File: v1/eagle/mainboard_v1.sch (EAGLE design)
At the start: 8 parts

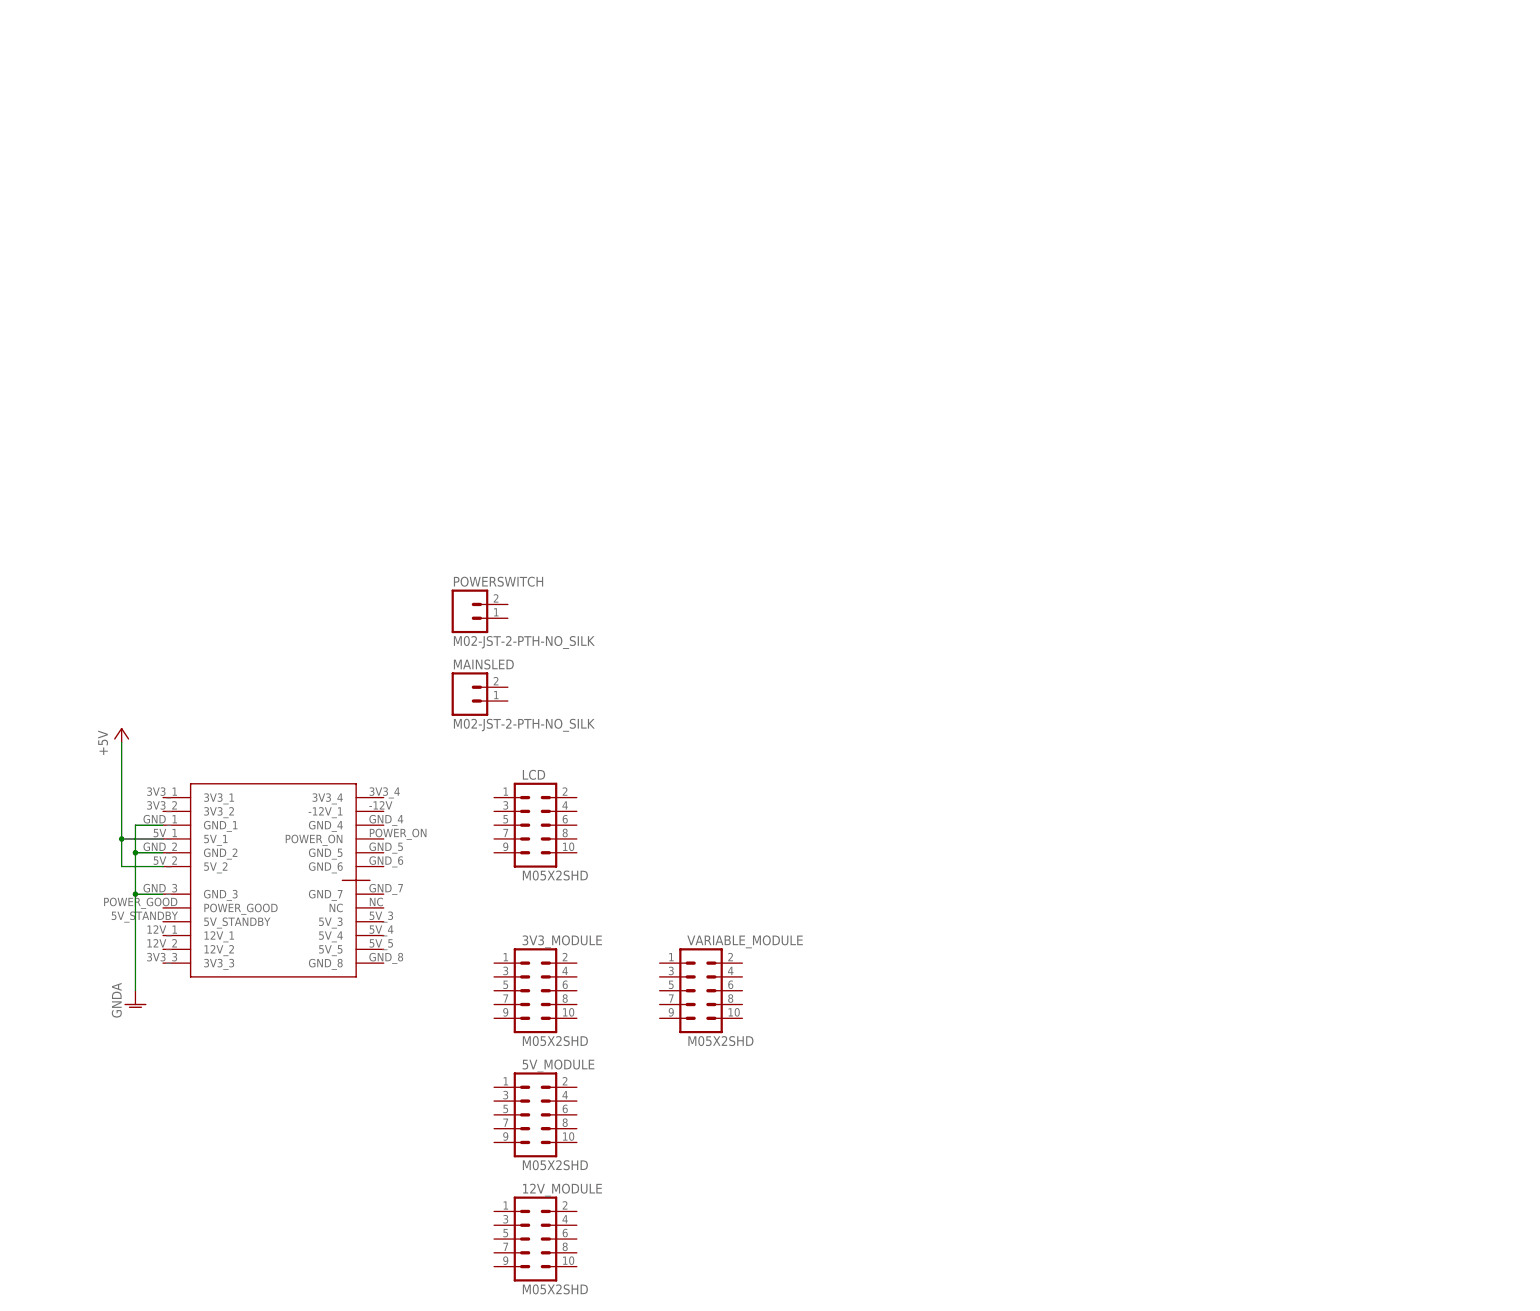
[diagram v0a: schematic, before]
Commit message: mainboard is all laid out
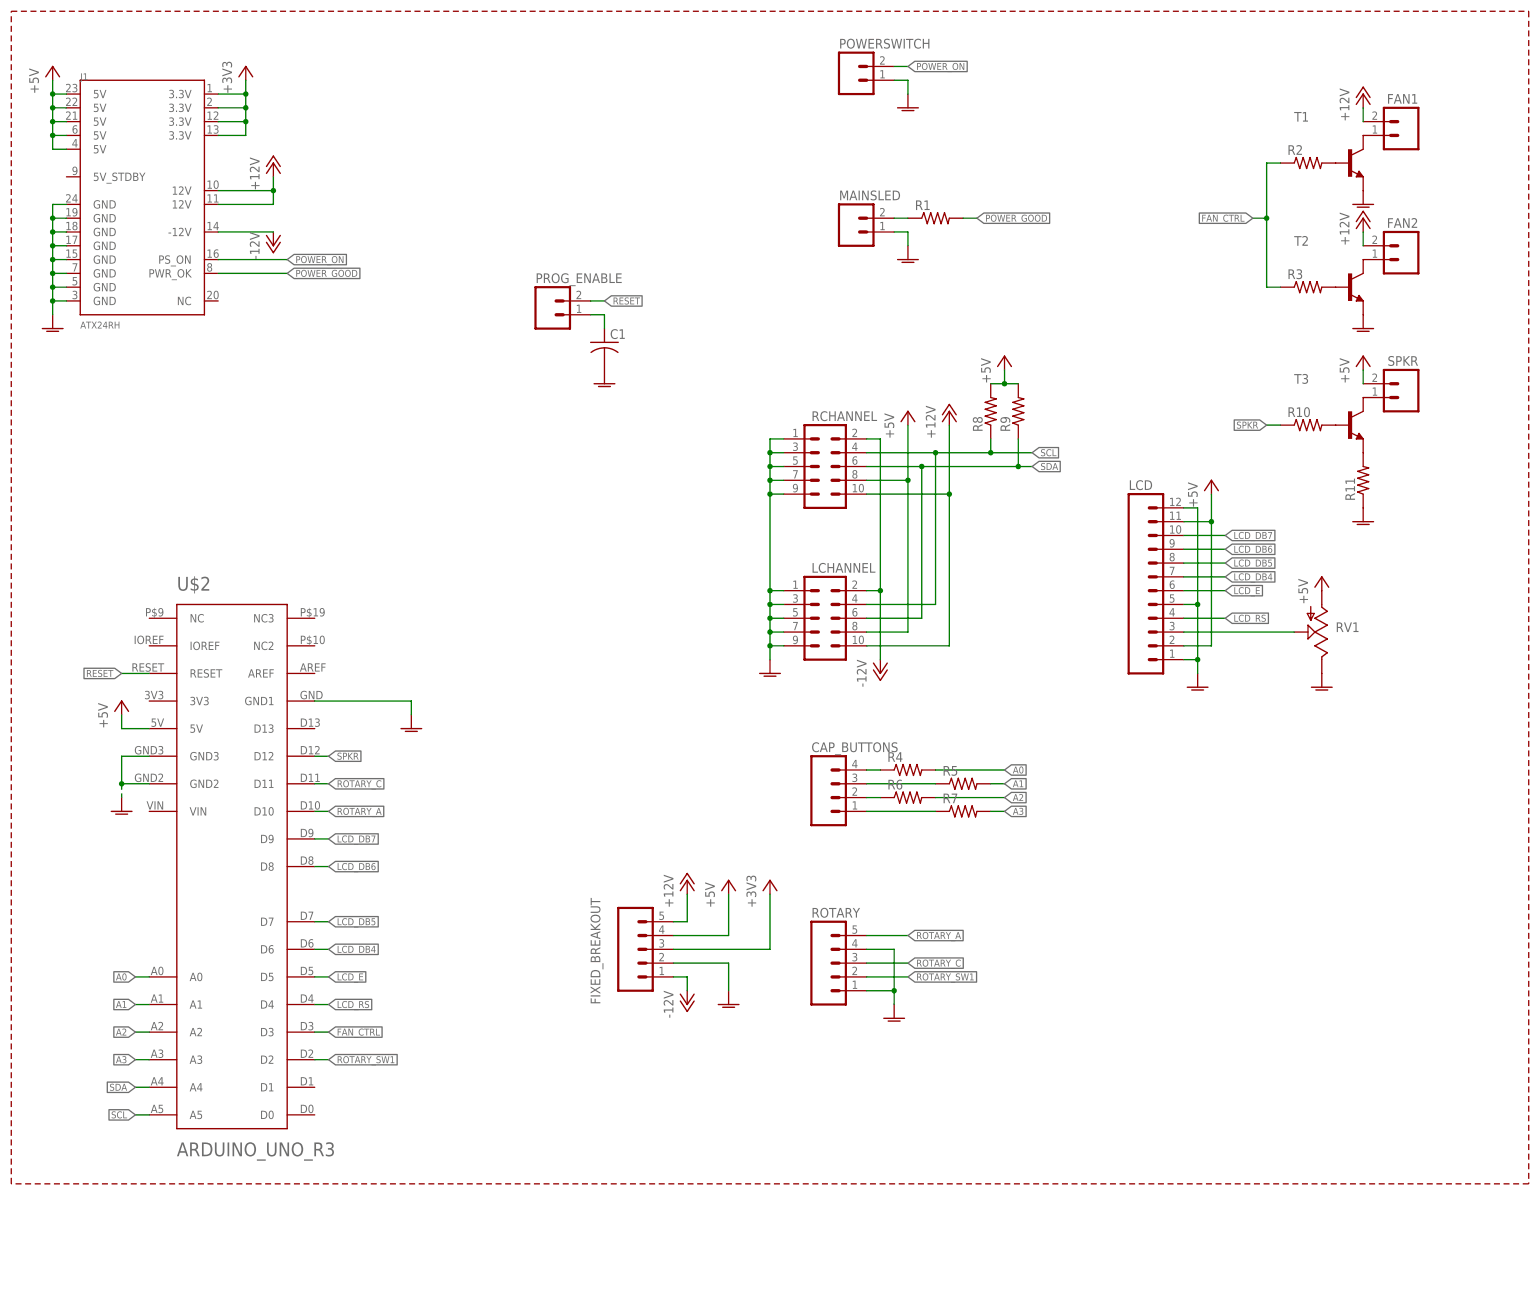
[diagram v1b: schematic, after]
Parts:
- removed 12V_MODULE, 3V3_MODULE, 5V_MODULE, VARIABLE_MODULE: M05X2SHD, SparkFun-Connectors:M05X2SHD
- removed U$1: ATX-PSU-24, parts:ATX-PSU-24
- added C1: (no value), rcl:C-USC0805
- added CAP_BUTTONS: (no value), con-amp-quick:M04
- added FAN1, FAN2, PROG_ENABLE, SPKR: M02PTH, SparkFun-Connectors:M02PTH
- added FIXED_BREAKOUT, ROTARY: (no value), con-amp-quick:M05
- added J1: ATX24RH, SparkFun-Connectors:ATX24RH
- added LCHANNEL, RCHANNEL: M05X2SHD, SparkFun-Connectors:M05X2SHD
- added R1, R10, R11, R2, R3, R4, R5, R6, R7, R8, R9: (no value), rcl:R-US_R0805
- added RV1: (no value), SparkFun-Electromechanical:POTTRIM
- added T1, T2, T3: (no value), transistor:MMBT2222ALT1-NPN-SOT23-BEC
- added U$2: ARDUINO_UNO_R3, parts:ARDUINO_UNO_R3
- LCD: value M05X2SHD -> (none); device SparkFun-Connectors:M05X2SHD -> con-amp-quick:M12
- MAINSLED, POWERSWITCH: value M02-JST-2-PTH-NO_SILK -> M02PTH; device SparkFun-Connectors:M02-JST-2-PTH-NO_SILK -> SparkFun-Connectors:M02PTH
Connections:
- new net +12V: FAN1.2, FAN2.2, FIXED_BREAKOUT.5, J1.12V@0, J1.12V@1, LCHANNEL.10, RCHANNEL.10
- new net +3V3: FIXED_BREAKOUT.3, J1.3.3V@0, J1.3.3V@1, J1.3.3V@2, J1.3.3V@3
- new net -12V: FIXED_BREAKOUT.1, J1.-12V, LCHANNEL.2, RCHANNEL.2
- new net A0: R4.2, U$2.A0
- new net A1: R5.2, U$2.A1
- new net A2: R6.2, U$2.A2
- new net A3: R7.2, U$2.A3
- new net FAN_CTRL: R2.1, R3.1, U$2.D3
- new net LCD_DB4: LCD.7, U$2.D6
- new net LCD_DB5: LCD.8, U$2.D7
- new net LCD_DB6: LCD.9, U$2.D8
- new net LCD_DB7: LCD.10, U$2.D9
- new net LCD_E: LCD.6, U$2.D5
- new net LCD_RS: LCD.4, U$2.D4
- new net N$1: R2.2, T1.B
- new net N$11: CAP_BUTTONS.4, R4.1
- new net N$12: CAP_BUTTONS.3, R5.1
- new net N$13: CAP_BUTTONS.2, R6.1
- new net N$14: CAP_BUTTONS.1, R7.1
- new net N$15: SPKR.1, T3.C
- new net N$16: R10.2, T3.B
- new net N$17: R11.2, T3.E
- new net N$19: C1.1, PROG_ENABLE.1
- new net N$2: MAINSLED.2, R1.1
- new net N$3: R3.2, T2.B
- new net N$4: FAN1.1, T1.C
- new net N$5: FAN2.1, T2.C
- new net N$6: LCD.3, RV1.S
- new net POWER_GOOD: J1.PWR_OK, R1.2
- new net POWER_ON: J1.PS_ON, POWERSWITCH.2
- new net RESET: PROG_ENABLE.2, U$2.RESET
- new net ROTARY_A: ROTARY.5, U$2.D10
- new net ROTARY_C: ROTARY.3, U$2.D11
- new net ROTARY_SW1: ROTARY.2, U$2.D2
- new net SCL: LCHANNEL.4, R8.1, RCHANNEL.4, U$2.A5
- new net SDA: LCHANNEL.6, R9.1, RCHANNEL.6, U$2.A4
- new net SPKR: R10.1, U$2.D12
- net +5V: now also FIXED_BREAKOUT.4, J1.5V@0, J1.5V@1, J1.5V@2, J1.5V@3, J1.5V@4, LCD.11, LCD.2, LCHANNEL.8, R8.2, R9.2, RCHANNEL.8, RV1.A, SPKR.2, U$2.5V; no longer U$1.5V_1, U$1.5V_2
- net GNDA: now also C1.2, FIXED_BREAKOUT.2, J1.GND@0, J1.GND@1, J1.GND@2, J1.GND@3, J1.GND@4, J1.GND@5, J1.GND@6, J1.GND@7, LCD.1, LCD.12, LCD.5, LCHANNEL.1, LCHANNEL.3, LCHANNEL.5, LCHANNEL.7, LCHANNEL.9, MAINSLED.1, POWERSWITCH.1, R11.1, RCHANNEL.1, RCHANNEL.3, RCHANNEL.5, RCHANNEL.7, RCHANNEL.9, ROTARY.1, ROTARY.4, RV1.E, T1.E, T2.E, U$2.GND1, U$2.GND2, U$2.GND3; no longer U$1.GND_1, U$1.GND_2, U$1.GND_3
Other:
- moved on the sheet: MAINSLED, POWERSWITCH

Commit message: outstanding work
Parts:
- removed CAP_BUTTONS: (no value), con-amp-quick:M04
- removed FIXED_BREAKOUT: (no value), con-amp-quick:M05
- removed MAINSLED, POWERSWITCH: M02PTH, SparkFun-Connectors:M02PTH
- removed R4, R5, R6, R7: (no value), rcl:R-US_R0805
- removed RV1: (no value), SparkFun-Electromechanical:POTTRIM
- removed T1, T2, T3: (no value), transistor:MMBT2222ALT1-NPN-SOT23-BEC
- added -12V_OUT, 12V_OUT, 3V3_OUT, 5V_OUT, GND_FIX: TPPAD1-20, testpad:TPPAD1-20
- added CH1, CH2: (no value), led:LED5MM
- added I2C_EXTRA, JP1: M05X2NO_SILK, SparkFun-Connectors:M05X2NO_SILK
- added LD1, LD2, LD3, LD4: (no value), led:DUOLED-RG-A
- added PWRGOOD, PWRSW, STANDBY: M02PTH, SparkFun-Connectors:M02PTH
- added Q1, Q2, QA1, QA2, QA3, QB1, QB2, QB3, QC1, QC2, QC3, QD1, QD2, QD3: 2N7002L, parts:2N7002L
- added QD4, QD5: BSS84, transistor-small-signal:BSS84
- added R12, RB1, RB2, RB3, RB4, RC1, RC2, RC3, RC4, RD1, RD2, RD3, RD4, RD5: (no value), rcl:R-US_R0805
- added R13: 1R1 10W, resistor-power:RMNS-5
- added RA1: 10k, rcl:R-US_R0805
- added RA2: 470, rcl:R-US_R0805
- added RA3, RA4: 1M, rcl:R-US_R0805
- added U$1, U$3, U$4, U$5: MF-R300, parts:MF-R300
- added U$10, U$6, U$8, U$9: SPST, parts:SPST
- LCD: device con-amp-quick:M12 -> con-amp-quick:M04
- U$2: value ARDUINO_UNO_R3 -> ARDUINO_UNO_R3MINIMUM; device parts:ARDUINO_UNO_R3 -> parts:ARDUINO_UNO_R3MINIMUM
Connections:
- removed net A2: R6.2, U$2.A2
- removed net A3: R7.2, U$2.A3
- removed net N$11: CAP_BUTTONS.4, R4.1
- removed net N$12: CAP_BUTTONS.3, R5.1
- removed net N$6: LCD.3, RV1.S
- new net 5V_OUT: 5V_OUT.TP, QB2.G, QB3.G, RB4.1, U$3.2
- new net 5V_OUT1: 3V3_OUT.TP, QC2.G, QC3.G, RC4.1, U$4.2
- new net 5V_STANDBY: J1.5V_STDBY, R1.2
- new net CH1_SW: CH1.C, U$2.A3
- new net CH2_SW: CH2.C, U$2.A2
- new net D13: JP1.1, U$2.D13
- new net N$18: PWRGOOD.2, R12.1
- new net N$20: RA1.1, U$1.2, U$6.P$2
- new net N$21: LD3.CR, QC1.D
- new net N$22: LD3.A, RC2.1
- new net N$23: LD3.CG, QC2.D
- new net N$24: QD1.G, QD3.D, RD1.2, RD3.1
- new net N$25: QD5.D, RD1.1
- new net N$26: LD4.CR, QD1.D
- new net N$27: 12V_OUT.TP, QA2.G, QA3.G, RA4.1, U$1.1
- new net N$28: QB1.G, QB3.D, RB1.2, RB3.1
- new net N$29: RB1.1, U$3.1, U$8.P$2
- new net N$30: LD4.A, RD2.1
- new net N$31: QA1.G, QA3.D, RA1.2, RA3.1
- new net N$32: LD4.CG, QD2.D
- new net N$33: QC1.G, QC3.D, RC1.2, RC3.1
- new net N$34: RC1.1, U$4.1, U$9.P$2
- new net N$36: -12V_OUT.TP, QD4.G, U$5.2
- new net N$39: QD5.G, RD5.1, U$10.P$2, U$5.1
- new net N$40: QD2.G, QD3.G, QD4.D, RD4.1
- new net N$9: LD2.A, RB2.1
- net +12V: now also U$6.P$1; no longer FIXED_BREAKOUT.5
- net +3V3: now also U$9.P$1; no longer FIXED_BREAKOUT.3
- net +5V: now also LCD.4, QD4.S, QD5.S, R10.1, R11.1, R13.1, RA2.2, RB2.2, RC2.2, RD2.2, RD5.2, U$8.P$1; no longer FIXED_BREAKOUT.4, LCD.11, LCD.2, RV1.A
- net -12V: now also U$10.P$1; no longer FIXED_BREAKOUT.1
- net A0: no longer R4.2
- net A1: no longer R5.2
- net FAN_CTRL: now also Q2.G, R2.2; no longer R2.1, R3.1
- net GNDA: now also GND_FIX.TP, JP1.10, JP1.2, JP1.4, JP1.6, JP1.8, LCD.3, PWRGOOD.1, PWRSW.1, Q1.S, Q2.S, QA1.S, QA2.S, QA3.S, QB1.S, QB2.S, QB3.S, QC1.S, QC2.S, QC3.S, QD1.S, QD2.S, QD3.S, R13.2, R2.1, R3.1, RA3.2, RA4.2, RB3.2, RB4.2, RC3.2, RC4.2, RD3.2, RD4.2, STANDBY.1; no longer FIXED_BREAKOUT.2, LCD.1, LCD.12, LCD.5, MAINSLED.1, POWERSWITCH.1, R11.1, RV1.E, T1.E, T2.E
- net LCD_DB4: no longer LCD.7
- net LCD_DB5: no longer LCD.8
- net LCD_DB6: no longer LCD.9
- net LCD_DB7: no longer LCD.10
- net LCD_E: no longer LCD.6
- net LCD_RS: no longer LCD.4
- net N$1: now also FAN1.1, FAN2.1, Q2.D; no longer R2.2, T1.B
- net N$13: now also LD1.A, RA2.1; no longer CAP_BUTTONS.2, R6.1
- net N$14: now also LD1.CG, QA2.D; no longer CAP_BUTTONS.1, R7.1
- net N$15: now also LD1.CR, QA1.D; no longer SPKR.1, T3.C
- net N$16: now also LD2.CG, QB2.D; no longer R10.2, T3.B
- net N$17: now also LD2.CR, QB1.D; no longer R11.2, T3.E
- net N$2: now also STANDBY.2; no longer MAINSLED.2
- net N$3: now also Q1.D, SPKR.1; no longer R3.2, T2.B
- net N$4: now also CH1.A, R10.2; no longer FAN1.1, T1.C
- net N$5: now also CH2.A, R11.2; no longer FAN2.1, T2.C
- net POWER_GOOD: now also R12.2; no longer R1.2
- net POWER_ON: now also PWRSW.2; no longer POWERSWITCH.2
- net SCL: now also I2C_EXTRA.1, I2C_EXTRA.3, I2C_EXTRA.5, I2C_EXTRA.7, I2C_EXTRA.9, LCD.1
- net SDA: now also I2C_EXTRA.10, I2C_EXTRA.2, I2C_EXTRA.4, I2C_EXTRA.6, I2C_EXTRA.8, LCD.2
- net SPKR: now also Q1.G, R3.2; no longer R10.1
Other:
- moved on the sheet: C1, FAN1, FAN2, J1, LCHANNEL, PROG_ENABLE, R1, R10, R11, R2, R3, R8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
